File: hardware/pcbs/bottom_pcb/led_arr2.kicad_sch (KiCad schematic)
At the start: 116 parts, among them U10 TPIC6C595, U3 TPIC6C595, U4 TPIC6C595, U5 TPIC6C595, U6 TPIC6C595, U7 TPIC6C595, U8 TPIC6C595, U9 TPIC6C595

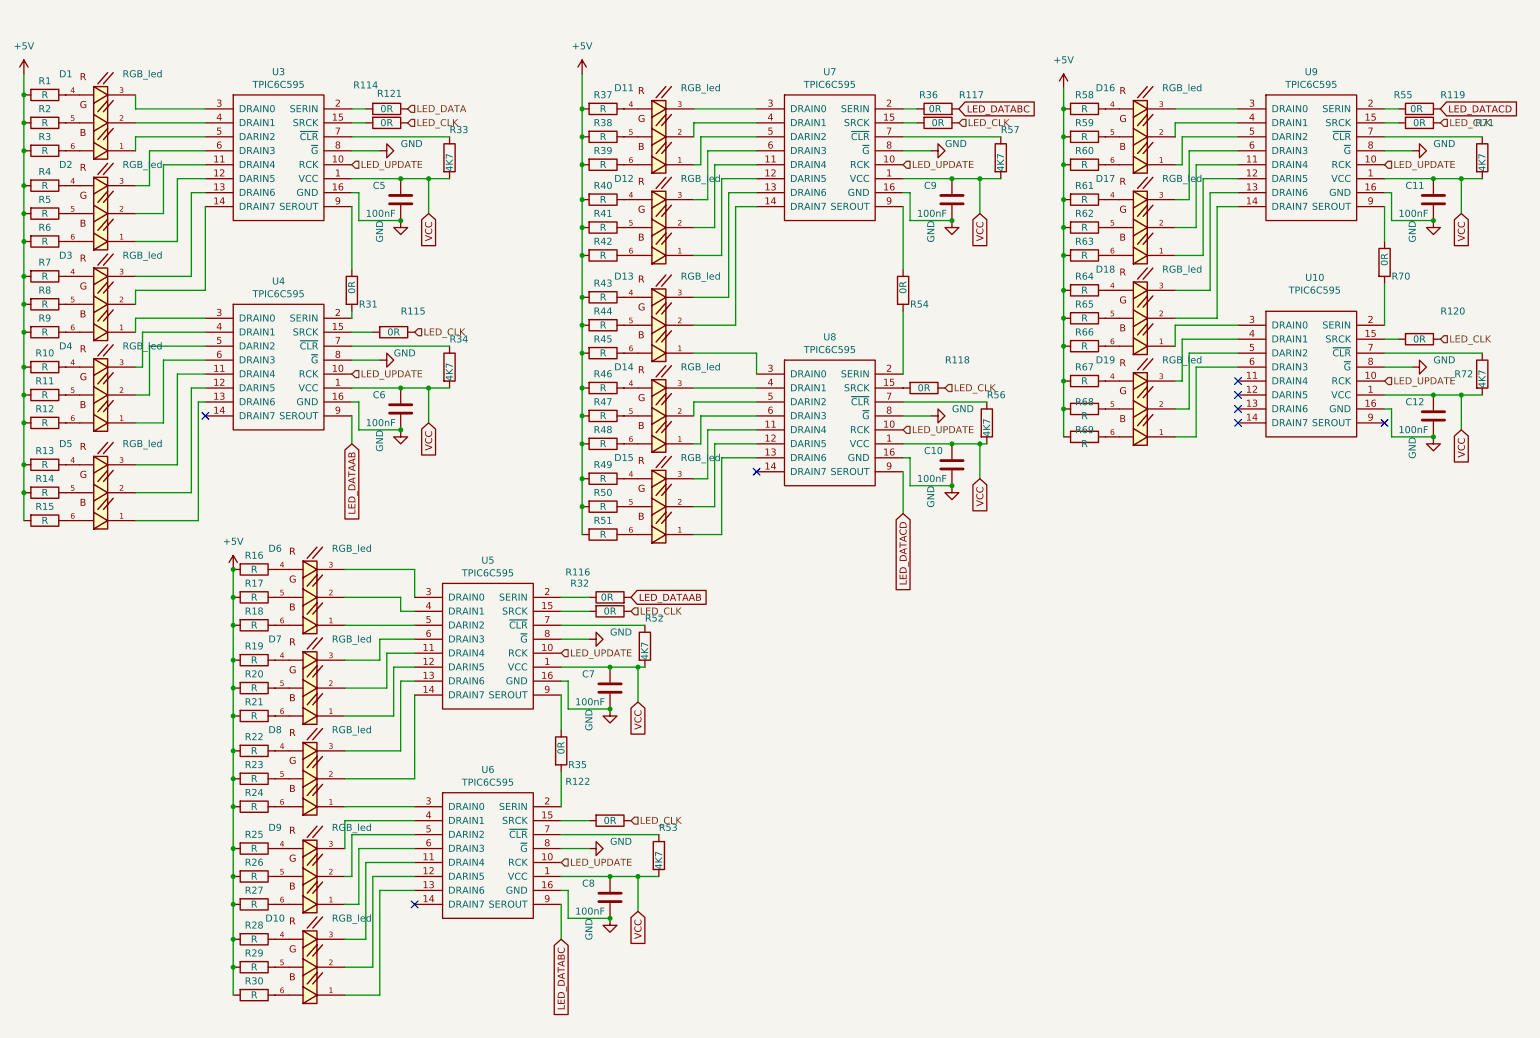
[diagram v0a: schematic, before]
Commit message: generated gerber files v31
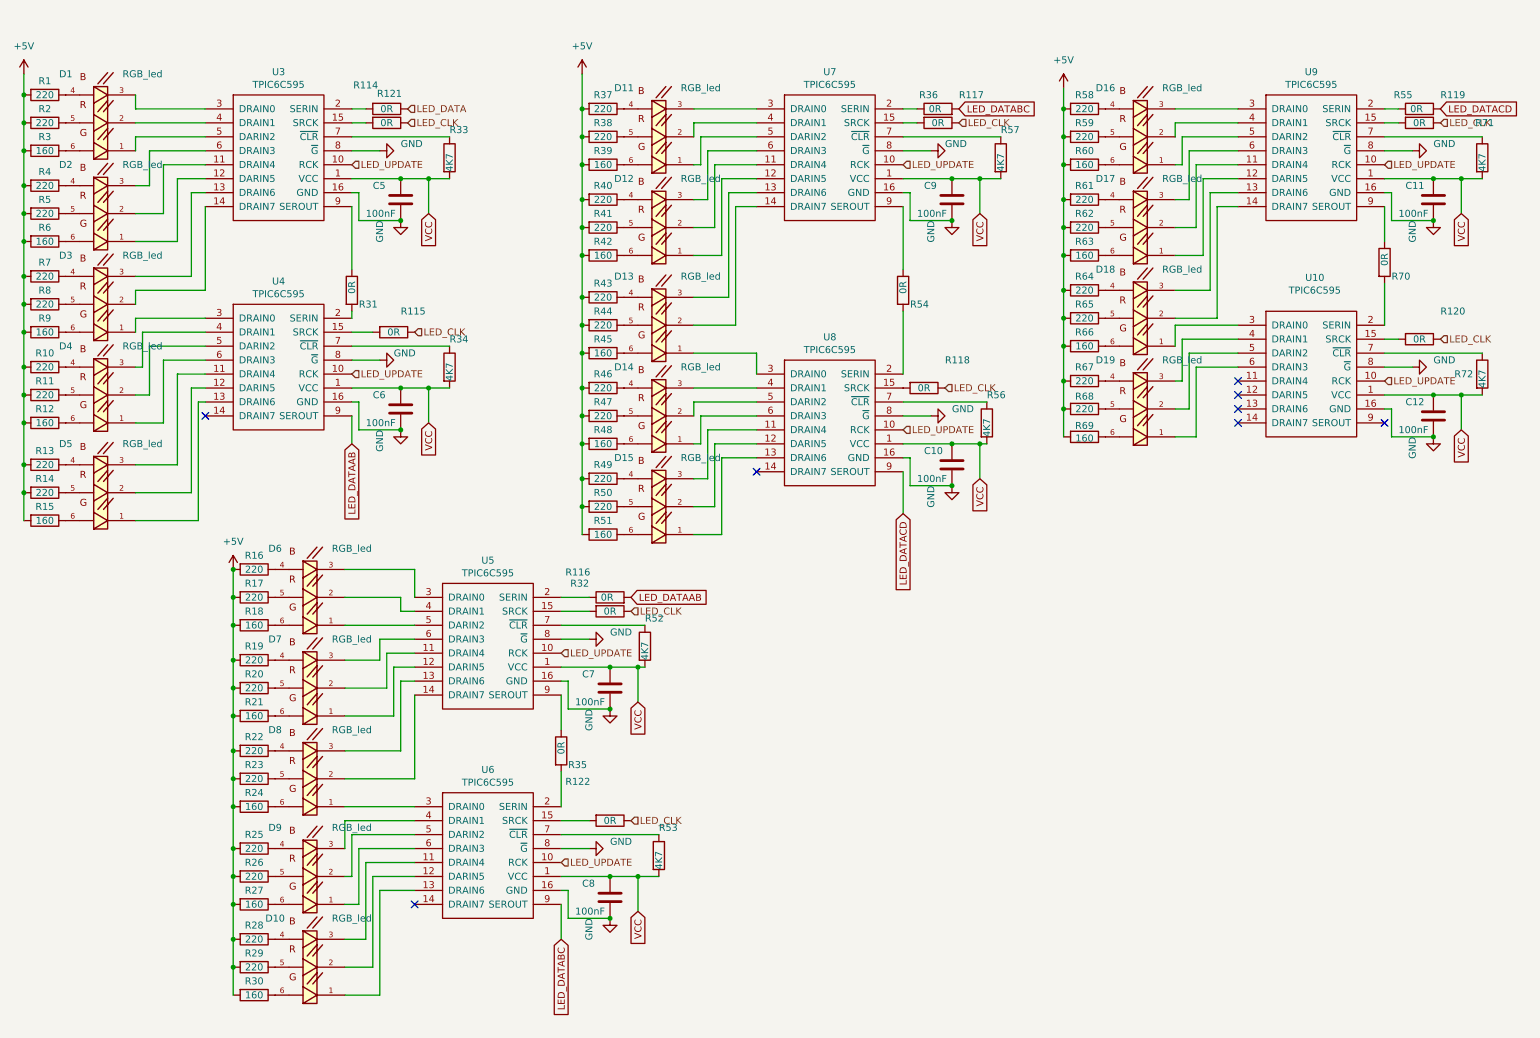
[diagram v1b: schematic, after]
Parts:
- R1, R10, R11, R13, R14, R16, R17, R19, R2, R20, R22, R23, R25, R26, R28, R29, R37, R38, R4, R40, R41, R43, R44, R46, R47, R49, R5, R50, R58, R59, R61, R62, R64, R65, R67, R68, R7, R8: value R -> 220
- R114, R115, R116, R117, R118, R119, R120, R121, R122, R31, R32, R33, R34, R35, R36, R52, R53, R54, R55, R56, R57, R70, R71, R72: footprint Resistor_SMD:R_1206_3216Metric_Pad1.30x1.75mm_HandSolder -> Resistor_SMD:R_1206_3216Metric
- R12, R15, R18, R21, R24, R27, R3, R30, R39, R42, R45, R48, R51, R6, R60, R63, R66, R69, R9: value R -> 160

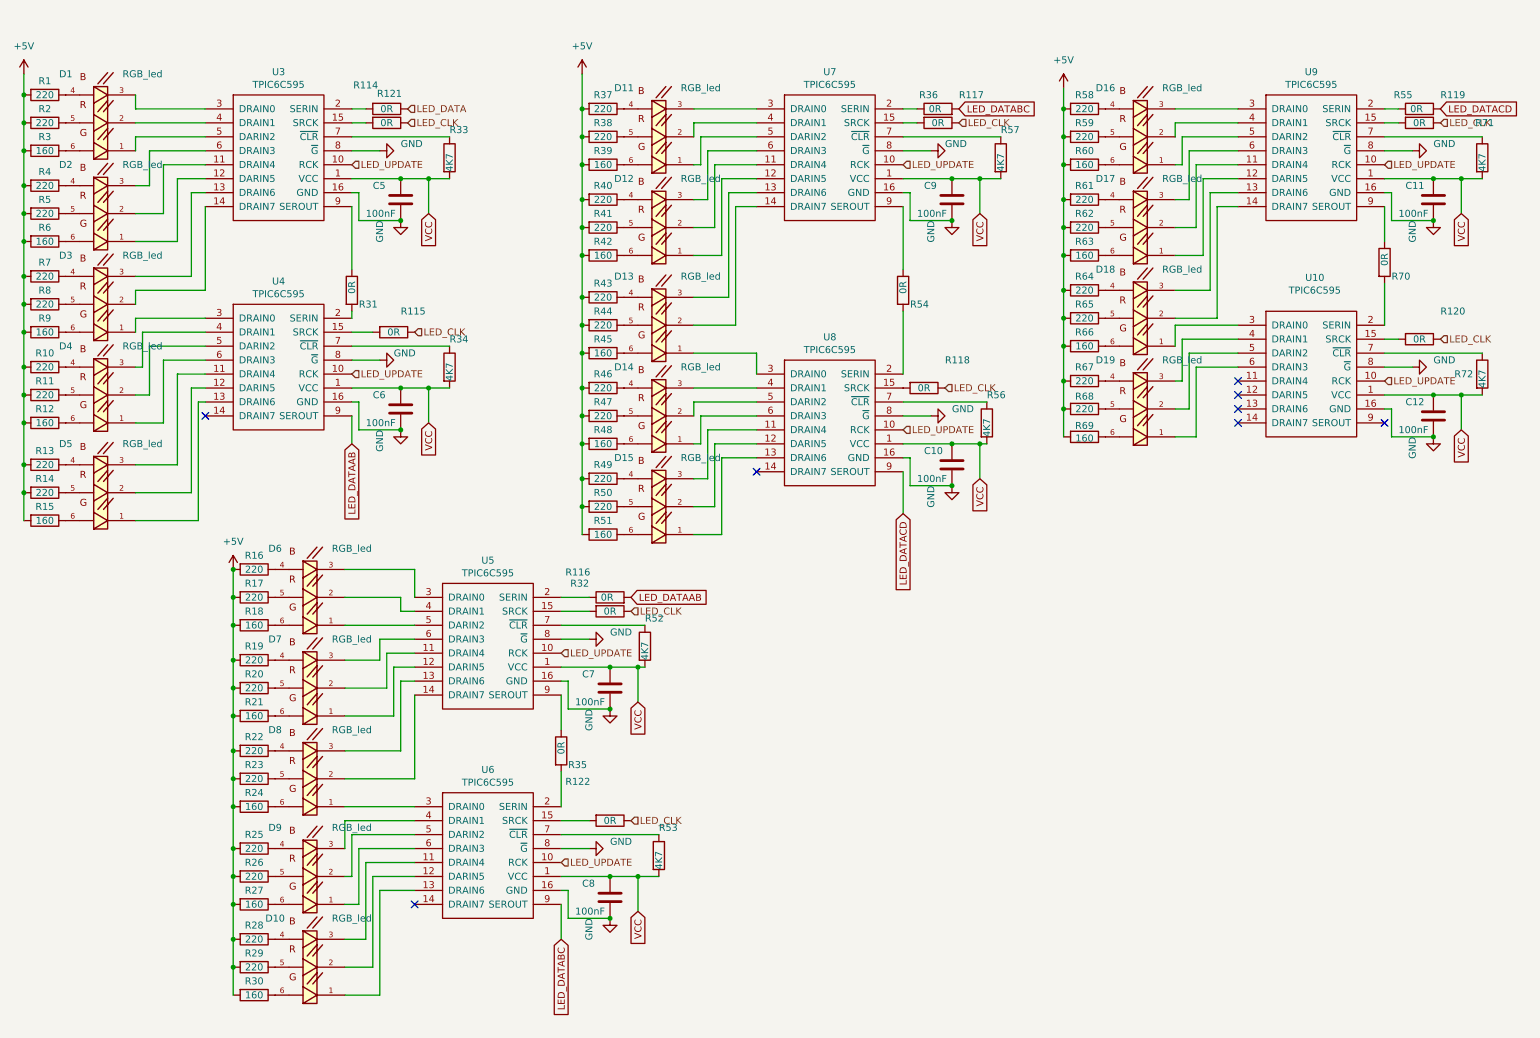
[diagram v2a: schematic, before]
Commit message: before ki
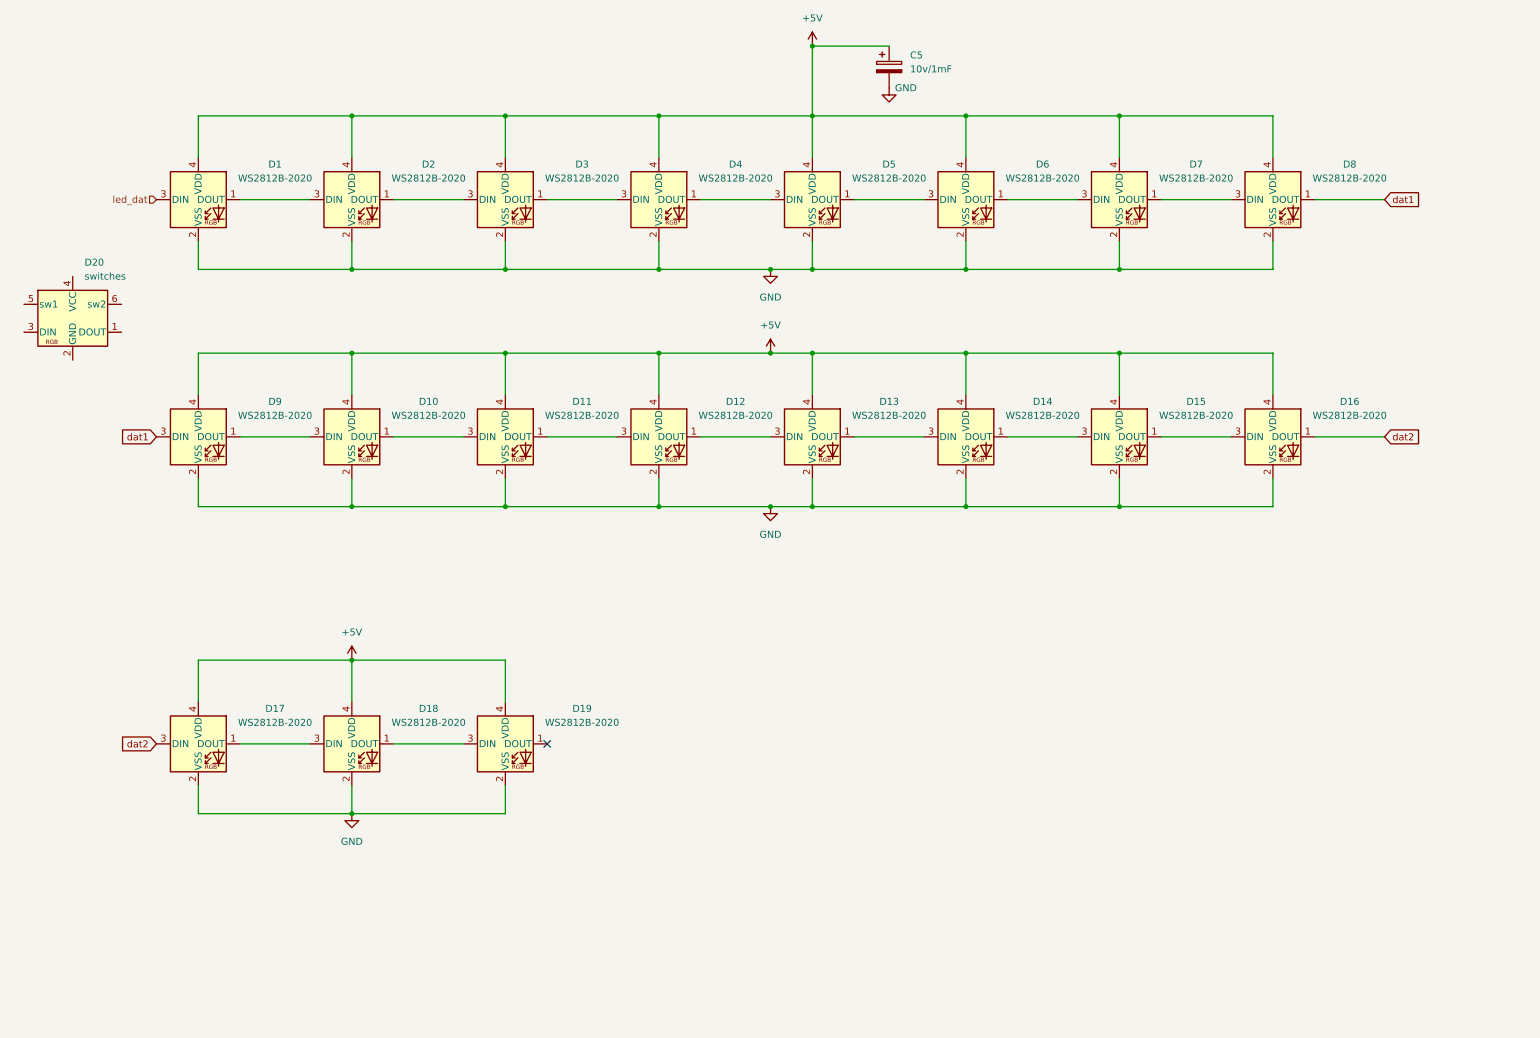
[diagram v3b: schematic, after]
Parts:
- removed C10, C11, C12, C5, C6, C7, C8, C9: 100nF, Capacitor_SMD:C_1206_3216Metric_Pad1.33x1.80mm_HandSolder, symbol Device:C
- removed D1, D10, D11, D12, D13, D14, D15, D16, D17, D18, D19, D2, D3, D4, D5, D6, D7, D8, D9: RGB_led, 3dAudioFoot:LED_QBLP679E-RGB, symbol 3dAudioSym:QBLP679E-RGB
- removed R1, R10, R11, R13, R14, R16, R17, R19, R2, R20, R22, R23, R25, R26, R28, R29, R37, R38, R4, R40, R41, R43, R44, R46, R47, R49, R5, R50, R58, R59, R61, R62, R64, R65, R67, R68, R7, R8: 220, Resistor_SMD:R_1206_3216Metric, symbol Device:R
- removed R114, R115, R116, R117, R118, R119, R120, R121, R122, R31, R32, R35, R36, R54, R55, R70: 0R, Resistor_SMD:R_1206_3216Metric, symbol Device:R
- removed R12, R15, R18, R21, R24, R27, R3, R30, R39, R42, R45, R48, R51, R6, R60, R63, R66, R69, R9: 160, Resistor_SMD:R_1206_3216Metric, symbol Device:R
- removed R33, R34, R52, R53, R56, R57, R71, R72: 4K7, Resistor_SMD:R_1206_3216Metric, symbol Device:R
- removed U10, U3, U4, U5, U6, U7, U8, U9: TPIC6C595, Package_SO:SOIC-16_3.9x9.9mm_P1.27mm, symbol 3dAudioSym:TPIC6C595
- added C5: 10v/1mF, Capacitor_SMD:CP_Elec_10x10, symbol Device:C_Polarized
- added D1, D10, D11, D12, D13, D14, D15, D16, D17, D18, D19, D2, D3, D4, D5, D6, D7, D8, D9: WS2812B-2020, LED_SMD:LED_WS2812B-2020_PLCC4_2.0x2.0mm, symbol LED:WS2812B-2020
- added D20: switches, 3dAudioFoot:A3_CherryMxHybrid_WS2812Led2020, symbol 3dAudioSym:A3_switches_led
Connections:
- net +5V: now also C5.1, D1.4 (VDD), D10.4 (VDD), D11.4 (VDD), D12.4 (VDD), D13.4 (VDD), D14.4 (VDD), D15.4 (VDD), D16.4 (VDD), D17.4 (VDD), D18.4 (VDD), D19.4 (VDD), D2.4 (VDD), D3.4 (VDD), D4.4 (VDD), D5.4 (VDD), D6.4 (VDD), D7.4 (VDD), D8.4 (VDD), D9.4 (VDD)
- net GND: now also C5.2, D1.2 (VSS), D10.2 (VSS), D11.2 (VSS), D12.2 (VSS), D13.2 (VSS), D14.2 (VSS), D15.2 (VSS), D16.2 (VSS), D17.2 (VSS), D18.2 (VSS), D19.2 (VSS), D2.2 (VSS), D3.2 (VSS), D4.2 (VSS), D5.2 (VSS), D6.2 (VSS), D7.2 (VSS), D8.2 (VSS), D9.2 (VSS)
- new net: D13.1 (DOUT), D14.3 (DIN)
- new net: D12.1 (DOUT), D13.3 (DIN)
- new net: D15.1 (DOUT), D16.3 (DIN)
- new net: D14.1 (DOUT), D15.3 (DIN)
- new net: D1.1 (DOUT), D2.3 (DIN)
- new net: D18.1 (DOUT), D19.3 (DIN)
- new net: D17.1 (DOUT), D18.3 (DIN)
- new net: D7.1 (DOUT), D8.3 (DIN)
- new net: D10.1 (DOUT), D11.3 (DIN)
- new net: D10.3 (DIN), D9.1 (DOUT)
- new net: D4.1 (DOUT), D5.3 (DIN)
- new net: D3.1 (DOUT), D4.3 (DIN)
- new net: D11.1 (DOUT), D12.3 (DIN)
- new net: D2.1 (DOUT), D3.3 (DIN)
- new net: D5.1 (DOUT), D6.3 (DIN)
- new net: D6.1 (DOUT), D7.3 (DIN)
- new net dat1: D8.1 (DOUT), D9.3 (DIN)
- new net dat2: D16.1 (DOUT), D17.3 (DIN)
- new net led_dat: D1.3 (DIN)
- no-connect marks 8 -> 1
